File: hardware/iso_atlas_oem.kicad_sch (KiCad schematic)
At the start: 4 parts, among them J2 Conn_Coaxial, J3 Conn_Coaxial, U3 Atlas Scientific OEM

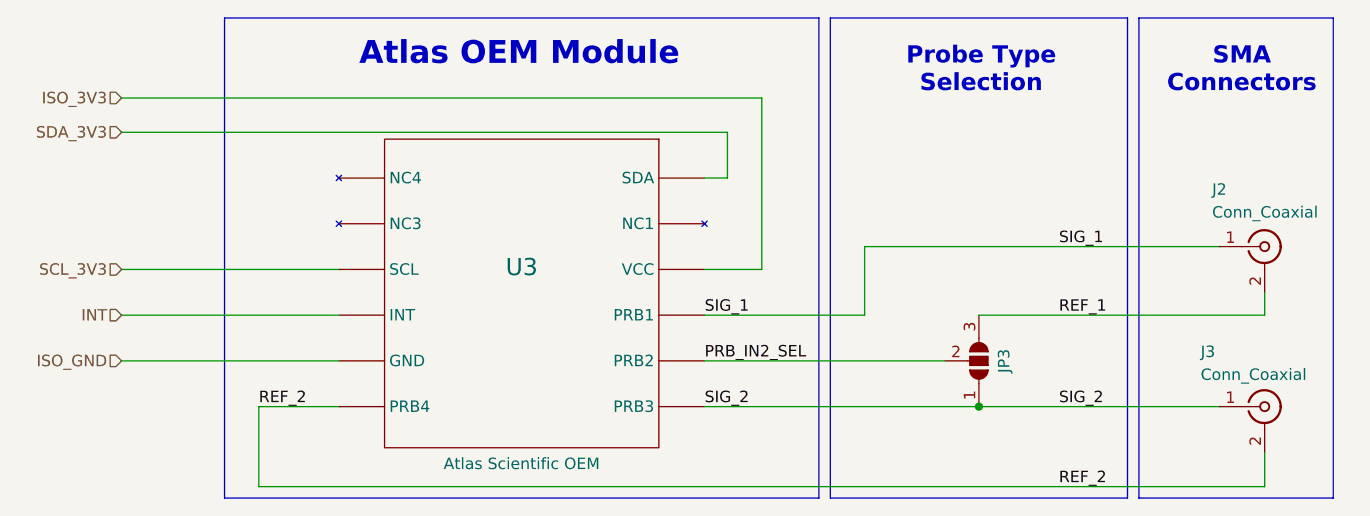
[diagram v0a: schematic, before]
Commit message: chores: clean up warnings and part references
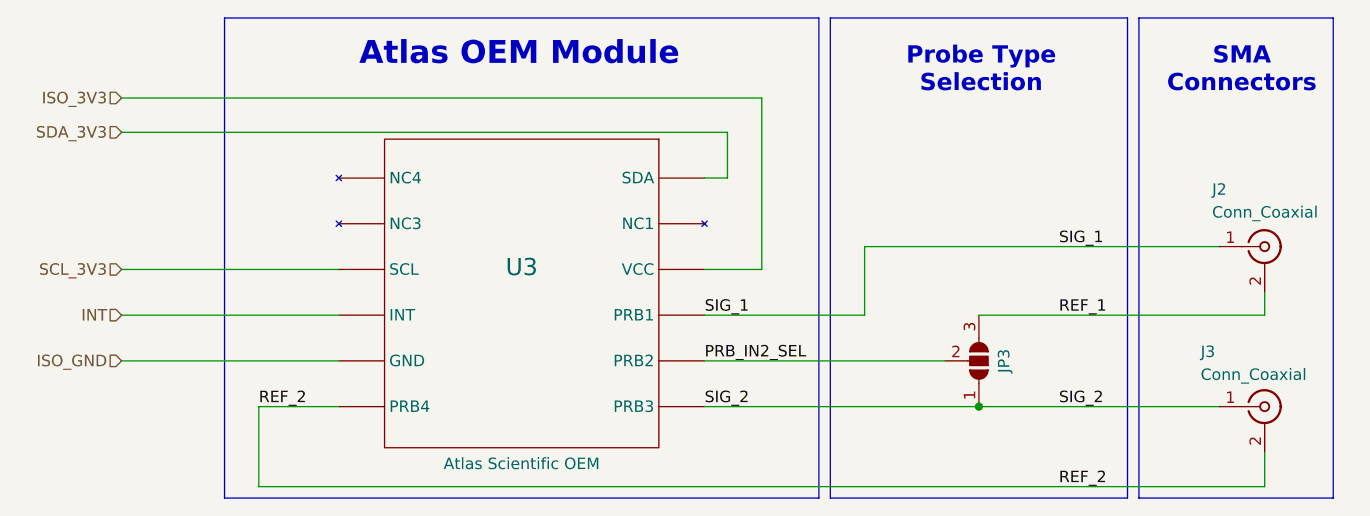
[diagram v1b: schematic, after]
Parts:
- U3: footprint kml-custom:Atlas_OEM -> KMLib_Boards_Modules:Atlas_OEM; symbol kml-custom:AtlasOEM -> KMLib_Sensors:AtlasOEM
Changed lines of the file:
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@@
 		)
 		(property "Datasheet" ""
-			(at 171.45 102.87 0)
+			(at 156.21 102.87 0)
 			(hide yes)
 			(show_name no)
@@
 		)
 		(property "Description" "Solder Jumper, 3-pole, open"
-			(at 171.45 102.87 0)
+			(at 158.75 102.87 0)
 			(hide yes)
 			(show_name no)
@@
 	)
 	(symbol
-		(lib_id "kml-custom:AtlasOEM")
+		(lib_id "KMLib_Sensors:AtlasOEM")
 		(at 120.65 92.71 0)
 		(mirror y)
@@
 			)
 		)
-		(property "Footprint" "kml-custom:Atlas_OEM"
+		(property "Footprint" "KMLib_Boards_Modules:Atlas_OEM"
 			(at 120.65 92.71 0)
 			(hide yes)
